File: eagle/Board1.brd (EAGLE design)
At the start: 160 x 100 mm, 7 parts

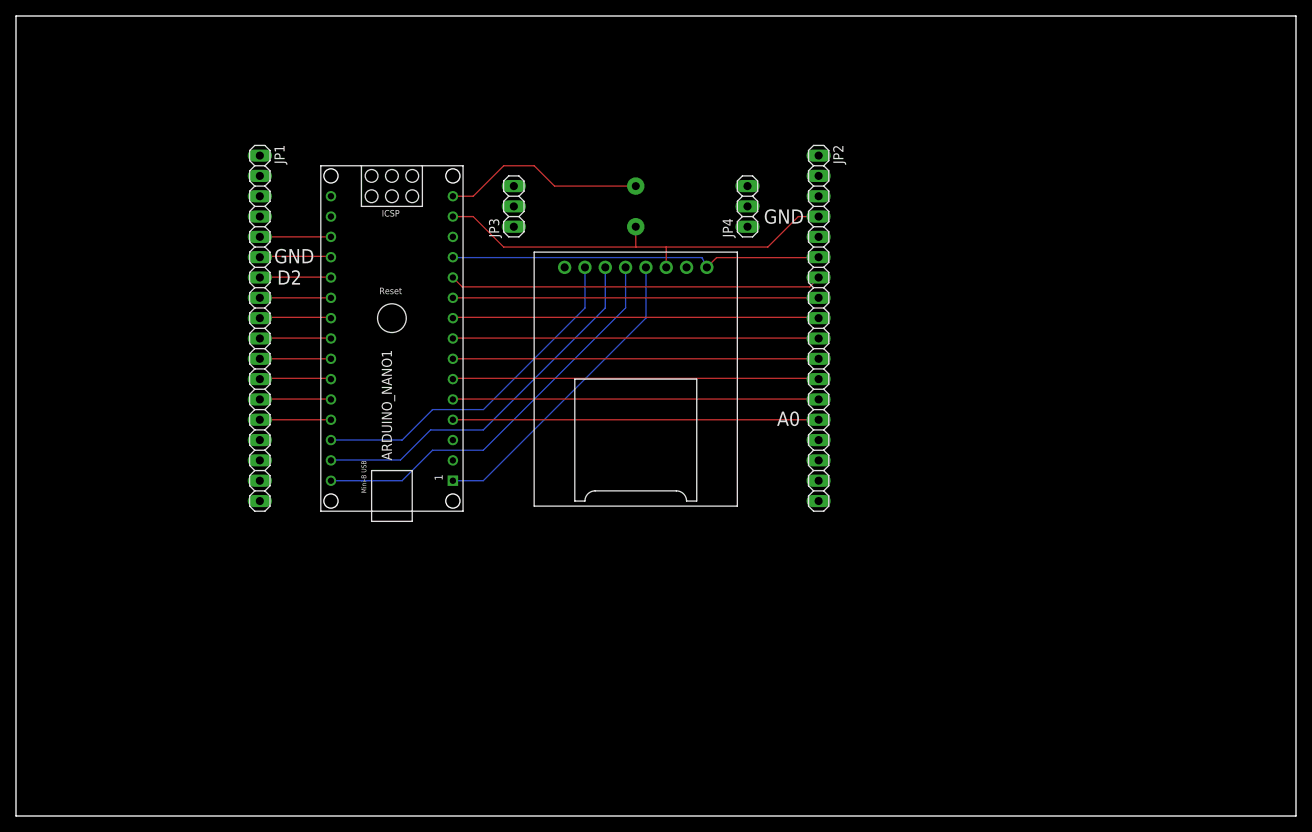
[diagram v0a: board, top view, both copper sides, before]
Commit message: Resize and tune board 1
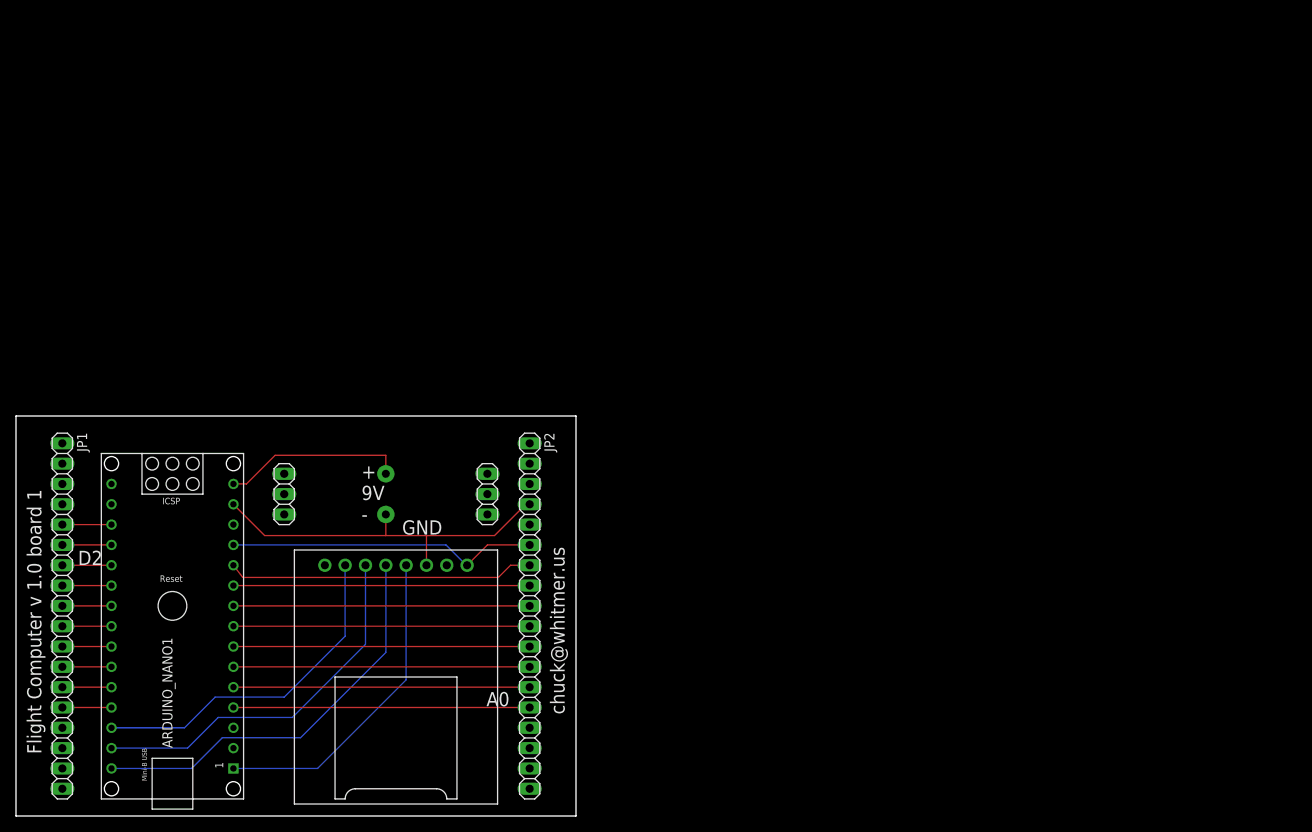
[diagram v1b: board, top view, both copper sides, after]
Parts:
- moved JP2 51.0 mm to (64.2, 25.0)
- moved JP4 48.5 mm to (58.9, 40.2)
- moved USD1 47.8 mm to (47.5, 17.4)
- moved BAT1 47.6 mm to (46.2, 40.2)
- moved JP3 46.0 mm to (33.5, 40.2)
- moved ARDUINO_NANO1 45.2 mm to (19.6, 26.3)
- moved JP1 43.6 mm to (5.79, 25.0)
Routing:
- net A5: track 45.8 -> 37.0 mm
- net A2: track 45.8 -> 37.0 mm
- net A4: track 45.8 -> 37.0 mm
- net A1: track 45.8 -> 37.0 mm
- net A6: track 45.7 -> 37.0 mm
- net A3: track 45.7 -> 37.0 mm
- net A0: track 45.7 -> 37.0 mm
- net A7: track 46.7 -> 38.4 mm
- net 5V: track 47.0 -> 39.1 mm
- net GND2: track 54.2 -> 46.6 mm
- net GND1: track 9.05 -> 6.15 mm
- net D4: track 9.05 -> 6.15 mm
- net D7: track 9.05 -> 6.15 mm
- net D8: track 8.96 -> 6.15 mm
- net D5: track 8.96 -> 6.15 mm
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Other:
- board size 160 x 100 mm -> 70 x 50 mm
- board text added: "+ 9V -"
- board text added: "Flight Computer v 1.0 board 1"
- board text added: "chuck@whitmer.us"
